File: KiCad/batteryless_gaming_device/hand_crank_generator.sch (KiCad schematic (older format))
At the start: 5 parts, among them M300 Hand Generator

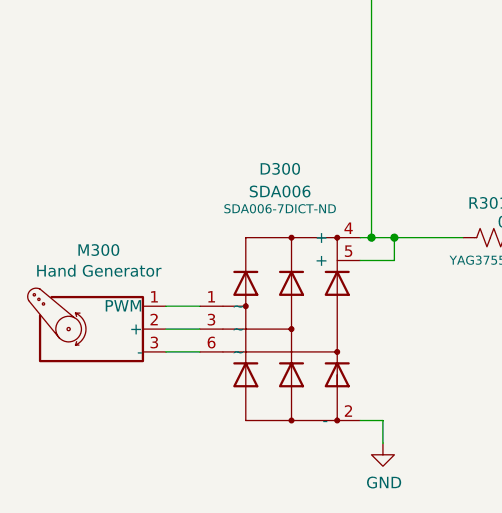
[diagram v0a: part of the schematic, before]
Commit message: oh ya
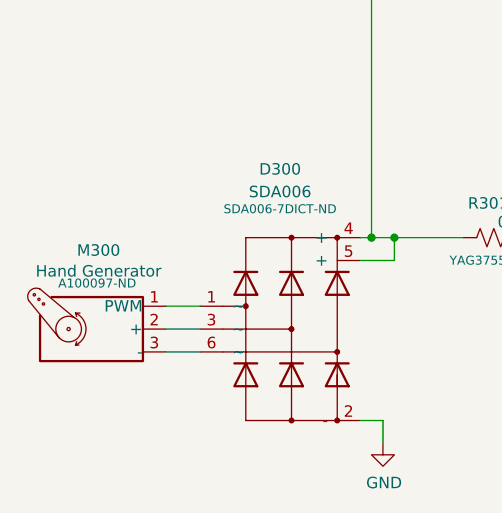
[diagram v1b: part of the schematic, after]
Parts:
- M300: footprint Connector_PinHeader_2.54mm:PinHeader_1x03_P2.54mm_Vertical -> Connector_PinHeader_2.00mm:PinHeader_1x03_P2.00mm_Vertical; Digikey PN (none) -> A100097-ND
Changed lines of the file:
@@
 F 0 "M300" H 4244 5244 50  0000 C CNN
 F 1 "Hand Generator" H 4244 5153 50  0000 C CNN
-F 2 "Connector_PinHeader_2.54mm:PinHeader_1x03_P2.54mm_Vertical" H 4250 4710 50  0001 C CNN
+F 2 "Connector_PinHeader_2.00mm:PinHeader_1x03_P2.00mm_Vertical" H 4250 4710 50  0001 C CNN
 F 3 "http://forums.parallax.com/uploads/attachments/46831/74481.png" H 4250 4710 50  0001 C CNN
+F 4 "A100097-ND" H 4250 5100 39  0000 C CNN "Digikey PN"
 	1    4250 4900
 	-1   0    0    -1

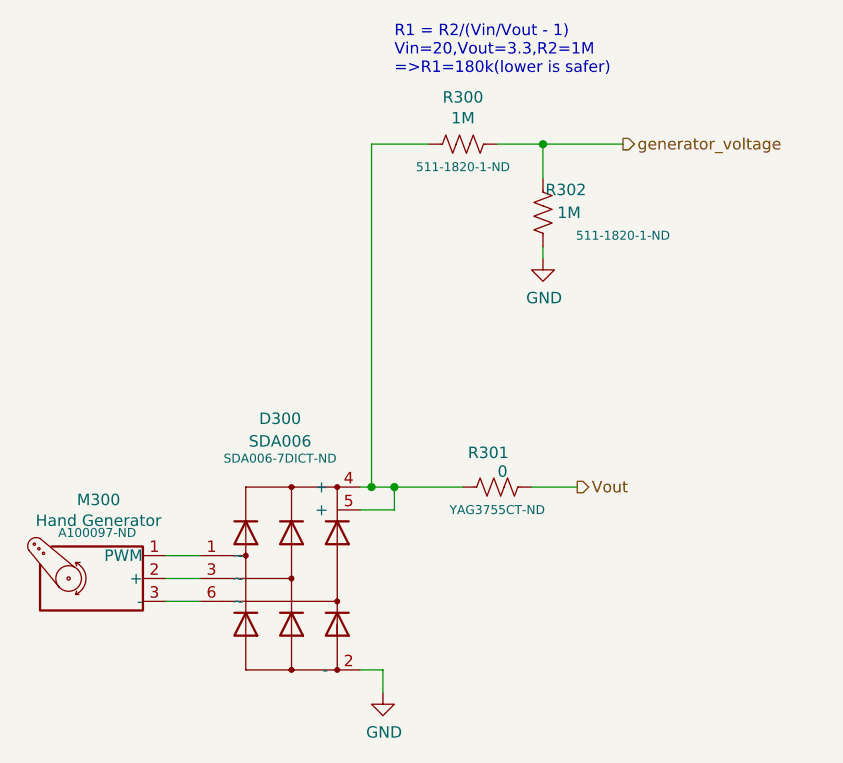
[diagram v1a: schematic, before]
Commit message: updated
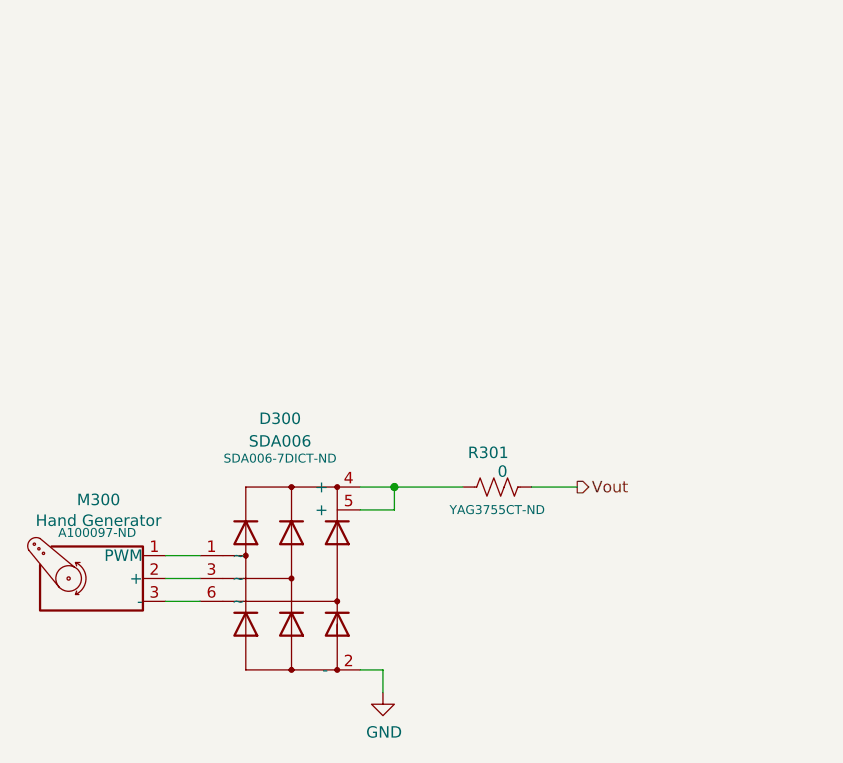
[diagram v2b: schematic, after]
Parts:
- removed R300, R302: 1M, Resistor_SMD:R_0603_1608Metric_Pad0.98x0.95mm_HandSolder, symbol Device:R_US
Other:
- note removed: "R1 = R2/(Vin/Vout - 1)\nVin=20,Vout=3.3,R2=1M\n=>R1=180k(lower is safer)"
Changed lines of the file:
@@
 Vout
-$Comp
-L Device:R_US R300
-U 1 1 6191BF70
-P 5850 3000
-F 0 "R300" V 5645 3000 50  0000 C CNN
-F 1 "1M" V 5736 3000 50  0000 C CNN
-F 2 "Resistor_SMD:R_0603_1608Metric_Pad0.98x0.95mm_HandSolder" V 5890 2990 50  0001 C CNN
-F 3 "~" H 5850 3000 50  0001 C CNN
-F 4 "511-1820-1-ND" V 5950 3000 39  0000 C CNN "Digikey PN"
-	1    5850 3000
-	0    1    1    0
-$EndComp
-Wire Wire Line
-	6200 3000 6000 3000
-Wire Wire Line
-	5400 4500 5450 4500
-Wire Wire Line
-	5450 4500 5450 3000
-Wire Wire Line
-	5450 3000 5700 3000
-Text Notes 5550 2700 0    50   ~ 0
-R1 = R2/(Vin/Vout - 1)\nVin=20,Vout=3.3,R2=1M\n=>R1=180k(lower is safer)
-Wire Wire Line
-	6200 3000 6550 3000
-Connection ~ 6200 3000
-Text HLabel 6550 3000 2    50   Output ~ 0
-generator_voltage
 $Comp
 L Device:R_US R?
@@
 Wire Wire Line
 	6150 4500 6350 4500
-Connection ~ 5450 4500
-Wire Wire Line
-	5450 4500 5550 4500
-$Comp
-L Device:R_US R302
-U 1 1 6196F794
-P 6200 3300
-F 0 "R302" H 6100 3200 50  0000 C CNN
-F 1 "1M" H 6086 3300 50  0000 C CNN
-F 2 "Resistor_SMD:R_0603_1608Metric_Pad0.98x0.95mm_HandSolder" V 6240 3290 50  0001 C CNN
-F 3 "~" H 6200 3300 50  0001 C CNN
-F 4 "511-1820-1-ND" H 5850 3400 39  0000 C CNN "Digikey PN"
-	1    6200 3300
-	-1   0    0    1
-$EndComp
-Wire Wire Line
-	6200 3000 6200 3150
-$Comp
-L power:GND #PWR0301
-U 1 1 619709AA
-P 6200 3500
-F 0 "#PWR0301" H 6200 3250 50  0001 C CNN
-F 1 "GND" H 6205 3327 50  0000 C CNN
-F 2 "" H 6200 3500 50  0001 C CNN
-F 3 "" H 6200 3500 50  0001 C CNN
-	1    6200 3500
-	1    0    0    -1
-$EndComp
-Wire Wire Line
-	6200 3450 6200 3500
 $Comp
 L batteryless_gaming_device-rescue:SDA006 D300
@@
 Wire Wire Line
 	5550 4500 5850 4500
+Wire Wire Line
+	5400 4500 5550 4500
 $EndSCHEMATC
